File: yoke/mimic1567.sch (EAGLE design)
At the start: 62 parts, among them J15 JST-VH-5, P1 25 K, P2 10 K, P4 20 K, P5 200, P6 44PINEDGE, Q1 2N3904, Q10 2N2907, Q12 2N3906, Q2 2N3904, Q3 2N3904, Q4 2N3904, Q5 2N3904, Q6 2N3904, Q7 2N3904, Q8 2N2907, Q9 2N3906

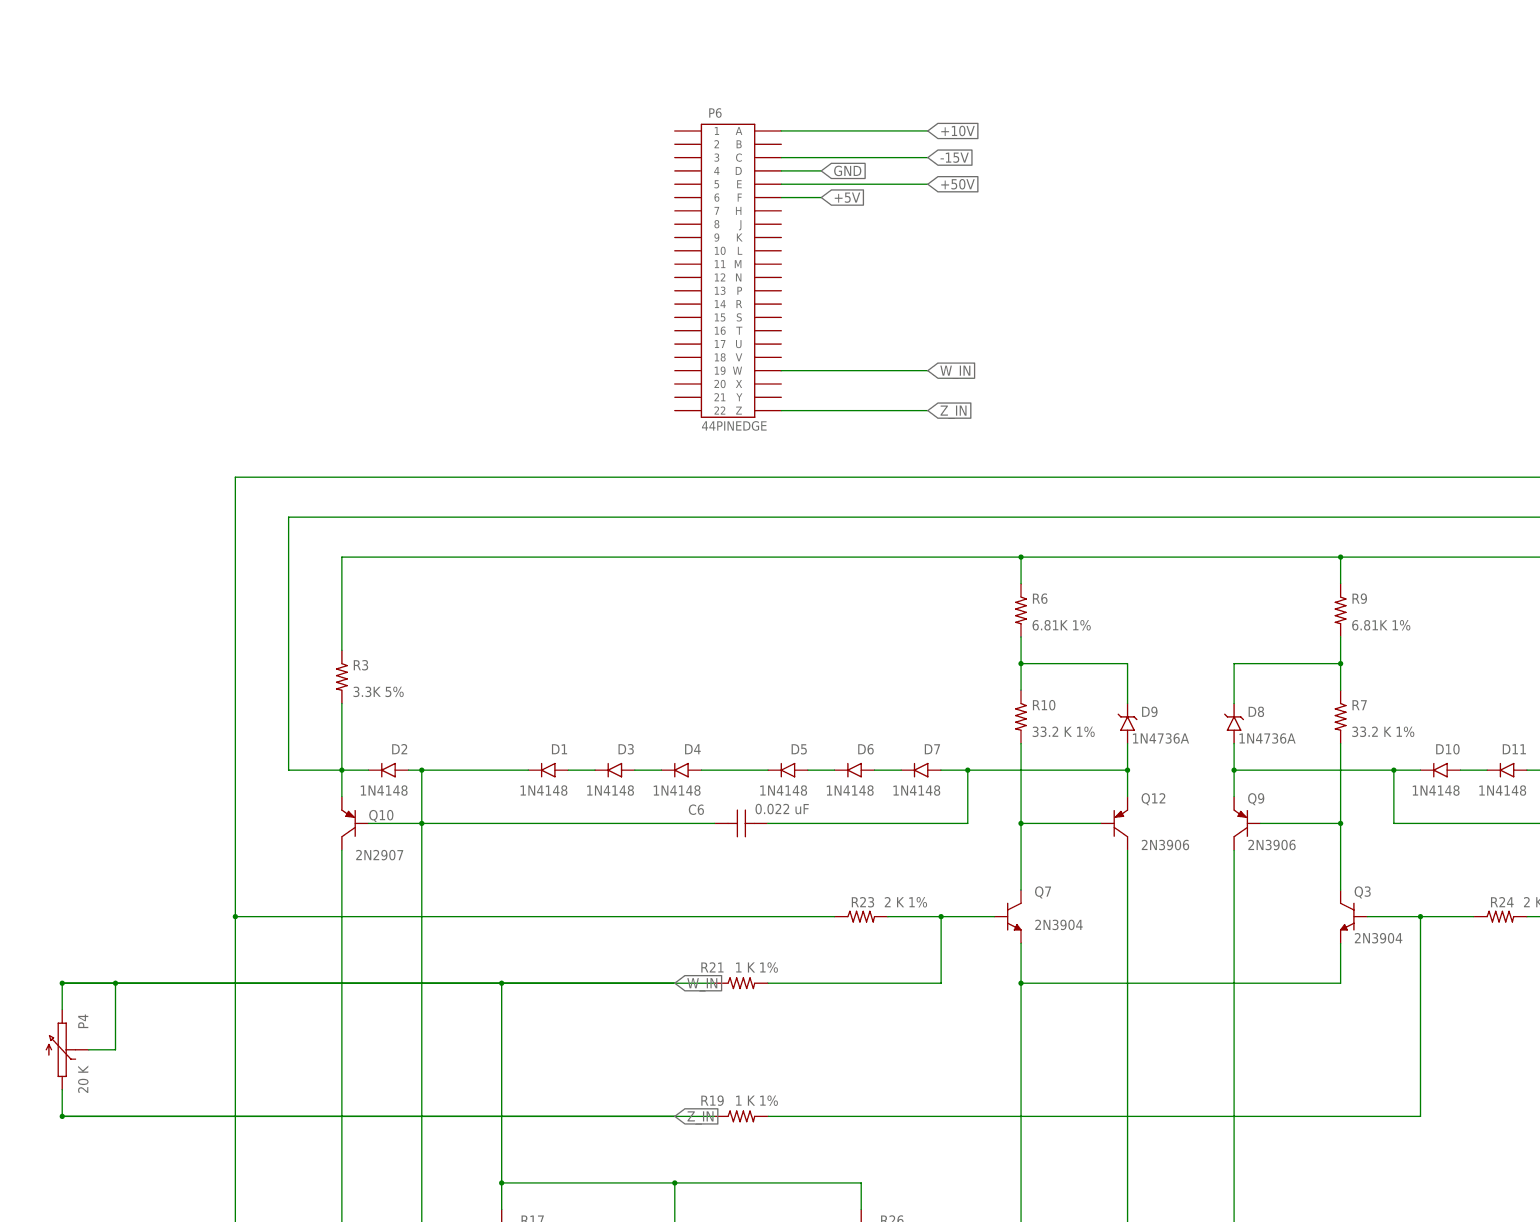
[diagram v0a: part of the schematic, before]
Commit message: update netlist
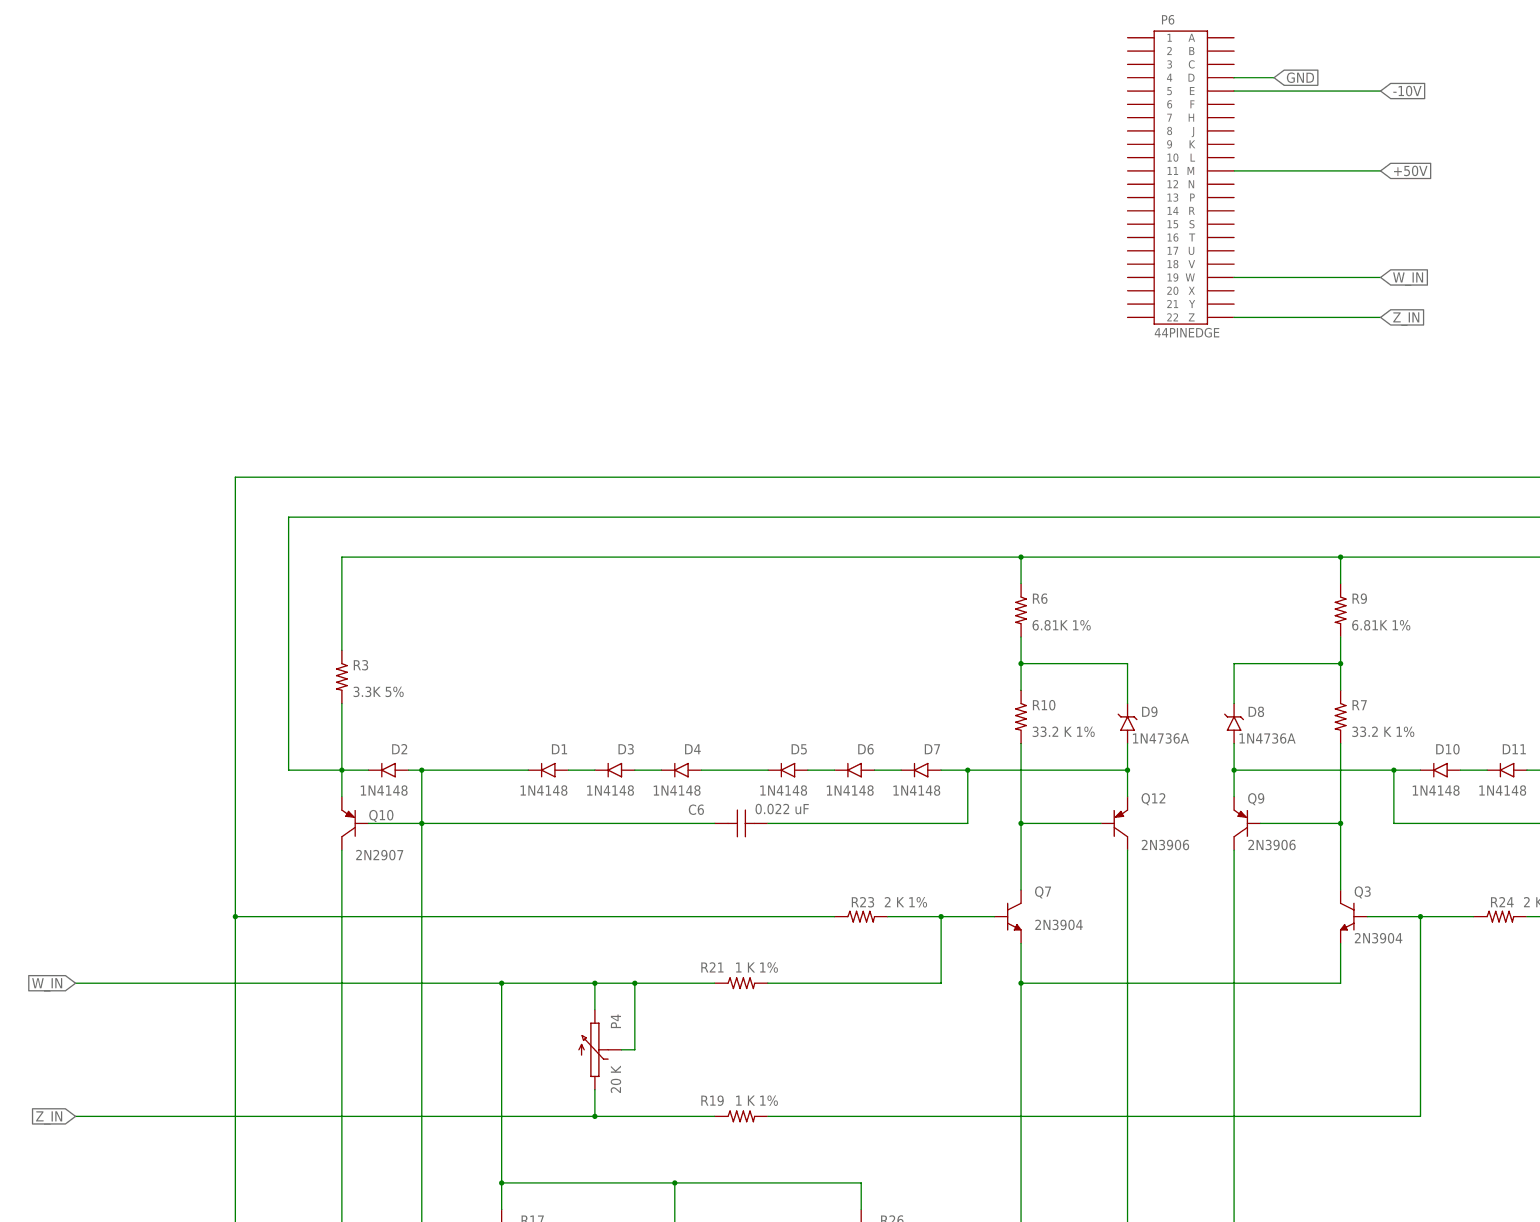
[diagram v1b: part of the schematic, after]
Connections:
- removed net +10V: P6.A
- removed net +5V: P6.F
- removed net -15V: P6.C
- net +50V: now also P6.M; no longer P6.E
- net -10V: now also P6.E
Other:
- moved on the sheet: P4, P6
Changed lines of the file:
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@@
 <attribute name="PN" x="165.1" y="101.6" size="1.778" layer="96" display="off"/>
 </instance>
-<instance part="P6" gate="G$1" x="208.28" y="335.28"/>
+<instance part="P6" gate="G$1" x="294.64" y="353.06"/>
 <instance part="R1" gate="G$1" x="391.16" y="129.54">
 <attribute name="PN" x="391.16" y="129.54" size="1.778" layer="96" display="off"/>
@@
 </instance>
 <instance part="SUPPLY2" gate="GND" x="403.86" y="106.68"/>
-<instance part="P4" gate="G$1" x="81.28" y="185.42" smashed="yes" rot="R90">
-<attribute name="NAME" x="84.328" y="192.278" size="1.9304" layer="95" font="vector" ratio="10" rot="R270"/>
-<attribute name="VALUE" x="84.328" y="182.372" size="1.9304" layer="96" font="vector" ratio="10" rot="R270"/>
-<attribute name="PN" x="81.28" y="185.42" size="1.778" layer="96" rot="R90" display="off"/>
+<instance part="P4" gate="G$1" x="182.88" y="185.42" smashed="yes" rot="R90">
+<attribute name="NAME" x="185.928" y="192.278" size="1.9304" layer="95" font="vector" ratio="10" rot="R270"/>
+<attribute name="VALUE" x="185.928" y="182.372" size="1.9304" layer="96" font="vector" ratio="10" rot="R270"/>
+<attribute name="PN" x="182.88" y="185.42" size="1.778" layer="96" rot="R90" display="off"/>
 </instance>
 <instance part="R21" gate="G$1" x="210.82" y="198.12" smashed="yes" rot="R90">
@@
 <pinref part="C5" gate="G$1" pin="1"/>
 </segment>
+<segment>
+<pinref part="P6" gate="G$1" pin="E"/>
+<wire x1="304.8" y1="368.3" x2="332.74" y2="368.3" width="0.1524" layer="91"/>
+<label x="332.74" y="368.3" size="1.9304" layer="95" font="vector" ratio="10" xref="yes"/>
+</segment>
 </net>
 <net name="N$22" class="0">
@@
 <pinref part="R17" gate="G$1" pin="P$2"/>
 <wire x1="165.1" y1="154.94" x2="165.1" y2="160.02" width="0.1524" layer="91"/>
-<wire x1="81.28" y1="198.12" x2="198.12" y2="198.12" width="0.1524" layer="91"/>
 <pinref part="P4" gate="G$1" pin="E"/>
-<wire x1="81.28" y1="193.04" x2="81.28" y2="198.12" width="0.1524" layer="91"/>
-<junction x="81.28" y="198.12"/>
-<wire x1="91.44" y1="198.12" x2="81.28" y2="198.12" width="0.1524" layer="91"/>
-<wire x1="91.44" y1="185.42" x2="91.44" y2="198.12" width="0.1524" layer="91"/>
+<wire x1="165.1" y1="198.12" x2="83.82" y2="198.12" width="0.1524" layer="91"/>
+<wire x1="190.5" y1="185.42" x2="190.5" y2="198.12" width="0.1524" layer="91"/>
 <pinref part="P4" gate="G$1" pin="S"/>
-<wire x1="86.36" y1="185.42" x2="91.44" y2="185.42" width="0.1524" layer="91"/>
-<label x="198.12" y="198.12" size="1.9304" layer="95" font="vector" ratio="10" xref="yes"/>
+<wire x1="187.96" y1="185.42" x2="190.5" y2="185.42" width="0.1524" layer="91"/>
+<label x="83.82" y="198.12" size="1.9304" layer="95" font="vector" ratio="10" rot="R180" xref="yes"/>
 <pinref part="R21" gate="G$1" pin="P$1"/>
-<junction x="91.44" y="198.12"/>
-<wire x1="205.74" y1="198.12" x2="165.1" y2="198.12" width="0.1524" layer="91"/>
+<junction x="190.5" y="198.12"/>
+<wire x1="205.74" y1="198.12" x2="190.5" y2="198.12" width="0.1524" layer="91"/>
 <pinref part="R26" gate="G$1" pin="P$2"/>
-<wire x1="165.1" y1="198.12" x2="91.44" y2="198.12" width="0.1524" layer="91"/>
+<wire x1="165.1" y1="198.12" x2="182.88" y2="198.12" width="0.1524" layer="91"/>
+<wire x1="182.88" y1="198.12" x2="190.5" y2="198.12" width="0.1524" layer="91"/>
 <wire x1="233.68" y1="154.94" x2="233.68" y2="160.02" width="0.1524" layer="91"/>
 <pinref part="P5" gate="G$1" pin="S"/>
@@
 <junction x="165.1" y="160.02"/>
 <junction x="165.1" y="198.12"/>
-</segment>
-<segment>
-<wire x1="218.44" y1="314.96" x2="246.38" y2="314.96" width="0.1524" layer="91"/>
-<label x="246.38" y="314.96" size="1.9304" layer="95" font="vector" ratio="10" xref="yes"/>
+<wire x1="182.88" y1="193.04" x2="182.88" y2="198.12" width="0.1524" layer="91"/>
+<junction x="182.88" y="198.12"/>
+</segment>
+<segment>
+<wire x1="304.8" y1="332.74" x2="332.74" y2="332.74" width="0.1524" layer="91"/>
+<label x="332.74" y="332.74" size="1.9304" layer="95" font="vector" ratio="10" xref="yes"/>
 <pinref part="P6" gate="G$1" pin="W"/>
 </segment>
@@
 <net name="Z_IN" class="0">
 <segment>
-<label x="198.12" y="172.72" size="1.9304" layer="95" font="vector" ratio="10" rot="MR180" xref="yes"/>
-<wire x1="81.28" y1="172.72" x2="198.12" y2="172.72" width="0.1524" layer="91"/>
+<label x="83.82" y="172.72" size="1.9304" layer="95" font="vector" ratio="10" rot="MR0" xref="yes"/>
 <pinref part="P4" gate="G$1" pin="A"/>
-<wire x1="81.28" y1="177.8" x2="81.28" y2="172.72" width="0.1524" layer="91"/>
-<junction x="81.28" y="172.72"/>
 <pinref part="R19" gate="G$1" pin="P$1"/>
-<wire x1="205.74" y1="172.72" x2="81.28" y2="172.72" width="0.1524" layer="91"/>
-</segment>
-<segment>
-<label x="246.38" y="307.34" size="1.9304" layer="95" font="vector" ratio="10" rot="MR180" xref="yes"/>
-<wire x1="218.44" y1="307.34" x2="246.38" y2="307.34" width="0.1524" layer="91"/>
+<wire x1="205.74" y1="172.72" x2="182.88" y2="172.72" width="0.1524" layer="91"/>
+<wire x1="182.88" y1="172.72" x2="83.82" y2="172.72" width="0.1524" layer="91"/>
+<wire x1="182.88" y1="177.8" x2="182.88" y2="172.72" width="0.1524" layer="91"/>
+<junction x="182.88" y="172.72"/>
+</segment>
+<segment>
+<label x="332.74" y="325.12" size="1.9304" layer="95" font="vector" ratio="10" rot="MR180" xref="yes"/>
+<wire x1="304.8" y1="325.12" x2="332.74" y2="325.12" width="0.1524" layer="91"/>
 <pinref part="P6" gate="G$1" pin="Z"/>
 </segment>
@@
 <segment>
 <pinref part="P6" gate="G$1" pin="D"/>
-<wire x1="218.44" y1="353.06" x2="226.06" y2="353.06" width="0.1524" layer="91"/>
-<label x="226.06" y="353.06" size="1.9304" layer="95" font="vector" ratio="10" xref="yes"/>
+<wire x1="304.8" y1="370.84" x2="312.42" y2="370.84" width="0.1524" layer="91"/>
+<label x="312.42" y="370.84" size="1.9304" layer="95" font="vector" ratio="10" xref="yes"/>
 </segment>
 <segment>
@@
 </segment>
 </net>
-<net name="-15V" class="0">
-<segment>
-<pinref part="P6" gate="G$1" pin="C"/>
-<wire x1="218.44" y1="355.6" x2="246.38" y2="355.6" width="0.1524" layer="91"/>
-<label x="246.38" y="355.6" size="1.9304" layer="95" font="vector" ratio="10" xref="yes"/>
-</segment>
-</net>
-<net name="+5V" class="0">
-<segment>
-<pinref part="P6" gate="G$1" pin="F"/>
-<wire x1="218.44" y1="347.98" x2="226.06" y2="347.98" width="0.1524" layer="91"/>
-<label x="226.06" y="347.98" size="1.9304" layer="95" font="vector" ratio="10" xref="yes"/>
-</segment>
-</net>
-<net name="+10V" class="0">
-<segment>
-<pinref part="P6" gate="G$1" pin="A"/>
-<wire x1="218.44" y1="360.68" x2="246.38" y2="360.68" width="0.1524" layer="91"/>
-<label x="246.38" y="360.68" size="1.9304" layer="95" font="vector" ratio="10" xref="yes"/>
-</segment>
-</net>
 <net name="+50V" class="0">
 <segment>
-<pinref part="P6" gate="G$1" pin="E"/>
-<wire x1="218.44" y1="350.52" x2="246.38" y2="350.52" width="0.1524" layer="91"/>
-<label x="246.38" y="350.52" size="1.9304" layer="95" font="vector" ratio="10" xref="yes"/>
-</segment>
-<segment>
+<label x="332.74" y="353.06" size="1.9304" layer="95" font="vector" ratio="10" xref="yes"/>
+<pinref part="P6" gate="G$1" pin="M"/>
+<wire x1="304.8" y1="353.06" x2="332.74" y2="353.06" width="0.1524" layer="91"/>
+</segment>
+<segment>
